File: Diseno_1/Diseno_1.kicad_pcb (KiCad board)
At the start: 2 copper layers, 114.3 x 108 mm, 71 parts, among them J1 Conn_01x06, Q1 MMBT3904, Q2 MMBT3904, Q3 MMBT3904, Q4 MMBT3904, U1 TPS563201, U2 TPS563201, U3 TPS563201, U4 TPS563201, U5 XC7Z010-BUENO, U6 MT41K256M16TW-107_P

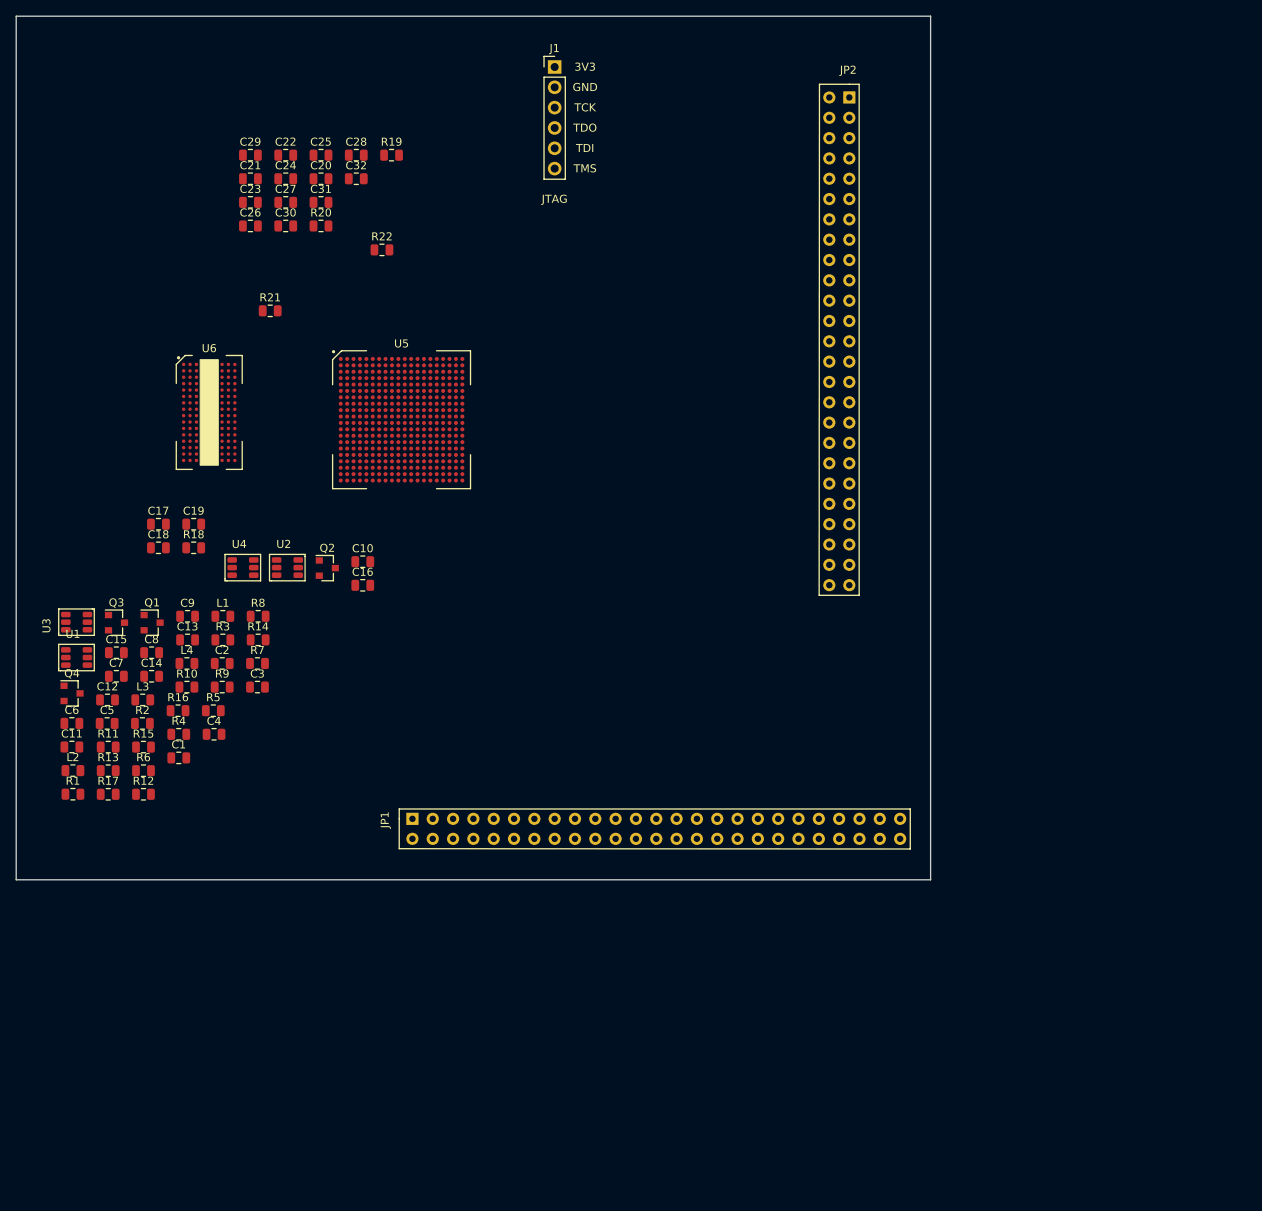
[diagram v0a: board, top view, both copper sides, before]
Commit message: actualizacion
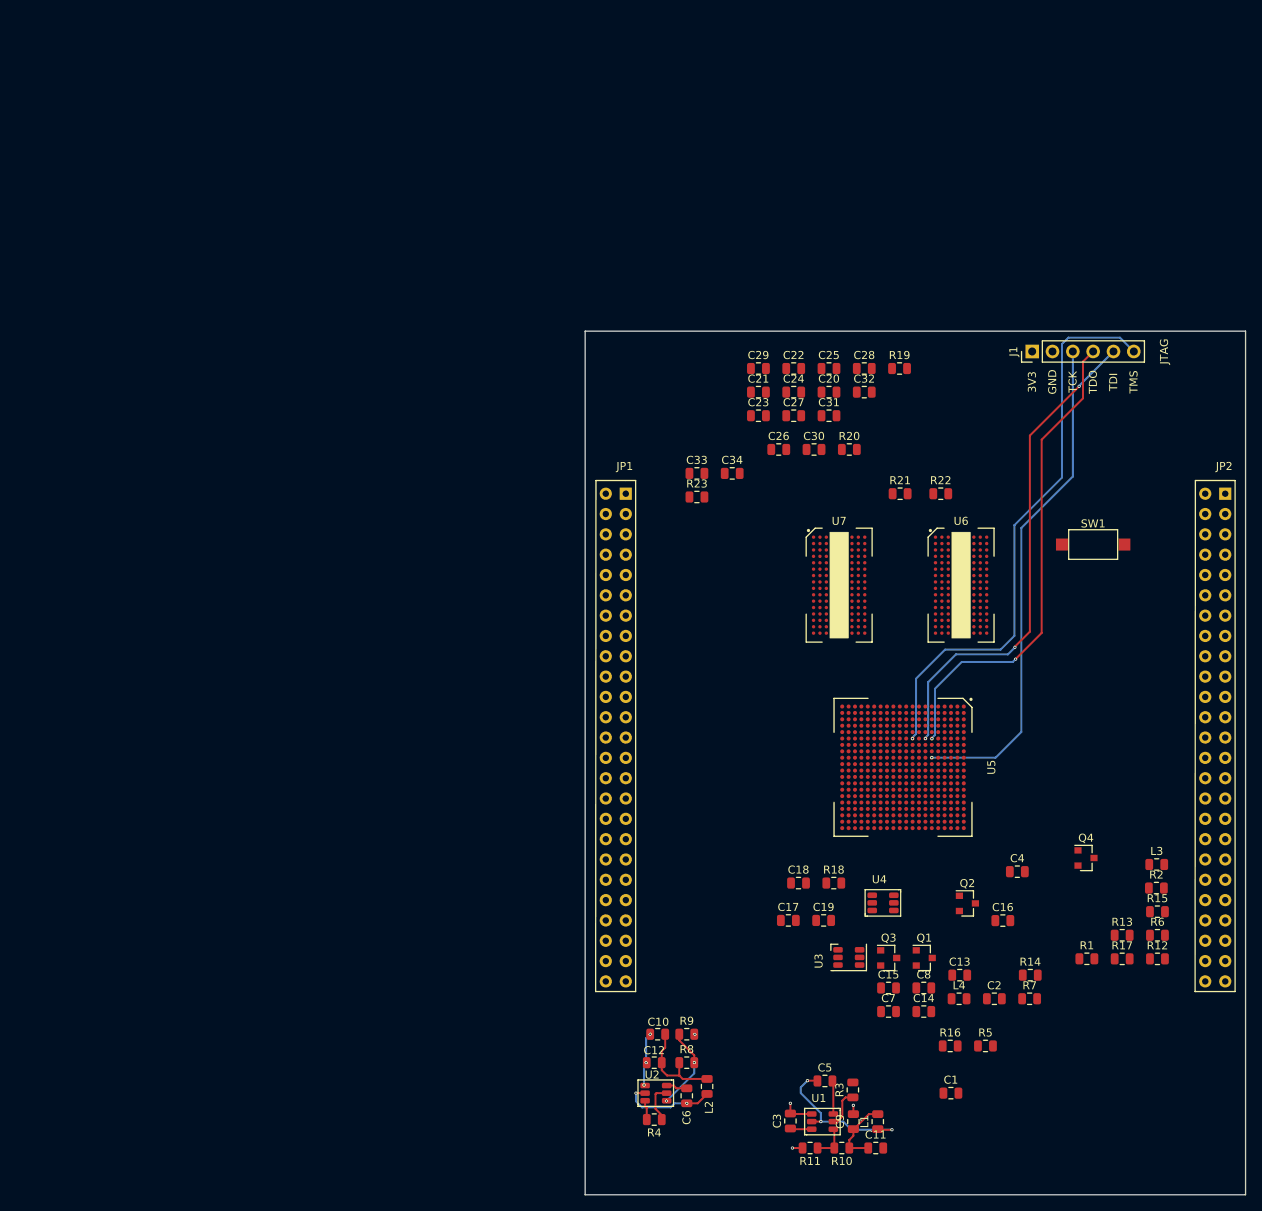
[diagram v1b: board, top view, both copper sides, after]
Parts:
- added C33: 100nF, Capacitor_SMD:C_0805_2012Metric, F.Cu at (153.7, 91.4)
- added C34: 100nF, Capacitor_SMD:C_0805_2012Metric, F.Cu at (158.1, 91.4)
- added R23: 240R 1%, Resistor_SMD:R_0805_2012Metric, F.Cu at (153.7, 94.4)
- added SW1: SW_Push, Button_Switch_SMD:SW_SPST_CK_RS282G05A3, F.Cu at (203.2, 100.3)
- added U7: MT41K256M16TW-107_P, ZYNQ_7000:BGA-144_9x16_8.0x14.0mm, F.Cu at (171.4, 105.4)
- moved Q4 128.4 mm to (202.3, 139.5)
- moved L3 128.4 mm to (211.1, 140.3)
- moved R1 128.4 mm to (202.4, 152.1)
- moved R12 128.4 mm to (211.2, 152.1)
- moved R13 128.4 mm to (206.8, 149.2)
- moved R15 128.4 mm to (211.2, 146.2)
- moved R17 128.4 mm to (206.8, 152.1)
- moved R2 128.4 mm to (211.1, 143.3)
- moved R6 128.4 mm to (211.2, 149.2)
- moved C11 112.3 mm to (176.0, 175.8)
- moved U1 109.8 mm to (169.4, 172.5)
- moved C13 105.2 mm to (186.5, 154.2)
- moved C15 105.2 mm to (177.6, 155.8)
- moved C7 105.2 mm to (177.6, 158.7)
- moved Q1 105.2 mm to (182.1, 152.0)
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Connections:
- JP1 pad 11: /Entradas y Salidas/BANK34_U13 -> (no net)
- U5 pad N5: (no net) -> /Memoria RAM/DDR_ODT
- U5 pad P1: (no net) -> /Memoria RAM/DDR_D16
- U5 pad P3: (no net) -> /Memoria RAM/DDR_D17
- U5 pad R1: (no net) -> /Memoria RAM/DDR_D19
- U5 pad R2: (no net) -> /Memoria RAM/DDR_DQS2+
- U5 pad R3: (no net) -> /Memoria RAM/DDR_D18
- U5 pad T1: (no net) -> /Memoria RAM/DDR_DQM2
- U5 pad T2: (no net) -> /Memoria RAM/DDR_DQS2-
- U5 pad T4: (no net) -> /Memoria RAM/DDR_D20
- U5 pad U13: /Entradas y Salidas/BANK34_U13 -> GND
- U5 pad U2: (no net) -> /Memoria RAM/DDR_D22
- U5 pad U3: (no net) -> /Memoria RAM/DDR_D23
- U5 pad U4: (no net) -> /Memoria RAM/DDR_D21
- U5 pad V1: (no net) -> /Memoria RAM/DDR_D24
- U5 pad V2: (no net) -> /Memoria RAM/DDR_D30
- U5 pad V3: (no net) -> /Memoria RAM/DDR_D31
- U5 pad W1: (no net) -> /Memoria RAM/DDR_D26
- U5 pad W3: (no net) -> /Memoria RAM/DDR_D29
- U5 pad W4: (no net) -> /Memoria RAM/DDR_DQS3-
- U5 pad W5: (no net) -> /Memoria RAM/DDR_DQS3+
- U5 pad Y1: (no net) -> /Memoria RAM/DDR_DQM3
- U5 pad Y2: (no net) -> /Memoria RAM/DDR_D28
- U5 pad Y3: (no net) -> /Memoria RAM/DDR_D25
- U5 pad Y4: (no net) -> /Memoria RAM/DDR_D27
- U6 pad K1: (no net) -> /Memoria RAM/DDR_ODT
- U6 pad L3: (no net) -> /Memoria RAM/DDR_WE
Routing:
- net /Referencias y MIOs/TMS: track 0.00 -> 71.2 mm, vias 0 -> 1
- net /Referencias y MIOs/TCK: track 0.00 -> 62.7 mm, vias 0 -> 1
- net /Referencias y MIOs/TDI: track 0.00 -> 61.9 mm, vias 0 -> 3
- net /Referencias y MIOs/TDO: track 0.00 -> 60.5 mm, vias 0 -> 2
- net Net-(C5-Pad1): track 0.00 -> 20.0 mm, vias 0 -> 3
- net GND: track 0.00 -> 13.0 mm, vias 0 -> 7
- net +1V0: track 0.00 -> 12.5 mm
- net Net-(C6-Pad1): track 0.00 -> 12.1 mm, vias 0 -> 2
- net Net-(R8-Pad2): track 0.00 -> 10.6 mm, vias 0 -> 2
- net +1V35: track 0.00 -> 8.76 mm
- net Net-(R3-Pad1): track 0.00 -> 5.38 mm
- net VCC: track 0.00 -> 5.14 mm
- net Net-(R4-Pad1): track 0.00 -> 4.96 mm
- net Net-(R10-Pad2): track 0.00 -> 4.50 mm
- net Net-(C5-Pad2): track 0.00 -> 4.17 mm
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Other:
- board size 114.3 x 108 mm -> 82.6 x 108 mm
